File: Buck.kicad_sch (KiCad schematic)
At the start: 6 parts, among them U1501 XL1509

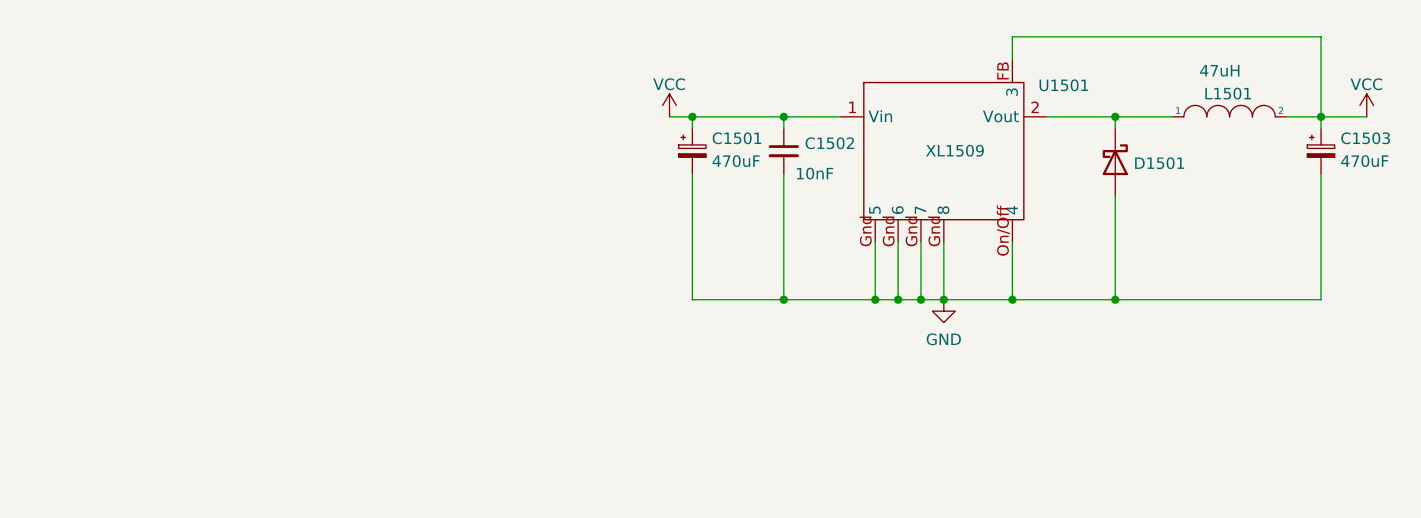
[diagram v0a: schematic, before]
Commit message: made additions to the project
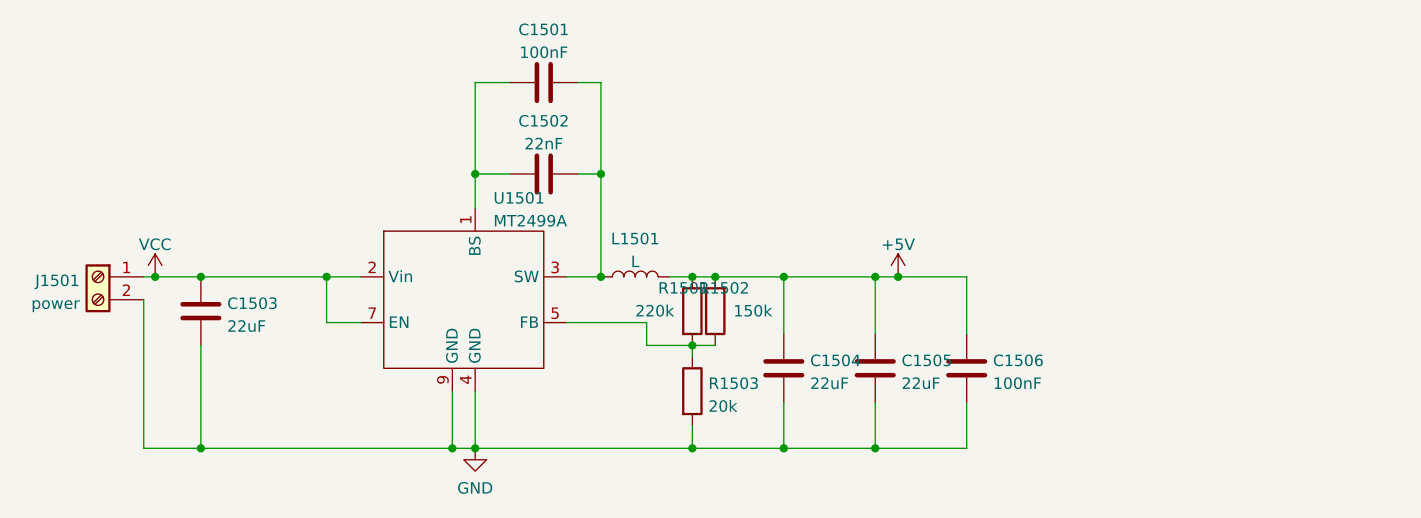
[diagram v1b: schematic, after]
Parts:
- removed C1501, C1503: 470uF, Capacitor_SMD:CP_Elec_8x10.5, symbol Device:C_Polarized_Small
- removed C1502: 10nF, Resistor_SMD:R_0805_2012Metric_Pad1.20x1.40mm_HandSolder, symbol Device:C_Small
- removed D1501: D_Schottky, Diode_SMD:D_SMA_Handsoldering, symbol Device:D_Schottky
- removed L1501: 47uH, Inductor_SMD:L_6.3x6.3_H3, symbol pspice:INDUCTOR
- removed U1501: XL1509, Package_SO:SOP-8_3.9x4.9mm_P1.27mm, symbol custom_bas:XL1509
- added C1501, C1506: 100nF, Capacitor_SMD:C_0402_1005Metric_Pad0.74x0.62mm_HandSolder, symbol Device:C
- added C1502: 22nF, Capacitor_SMD:C_0402_1005Metric_Pad0.74x0.62mm_HandSolder, symbol Device:C
- added C1503, C1504, C1505: 22uF, Capacitor_SMD:C_0603_1608Metric_Pad1.08x0.95mm_HandSolder, symbol Device:C
- added J1501: power, TerminalBlock_Phoenix:TerminalBlock_Phoenix_MKDS-1,5-2-5.08_1x02_P5.08mm_Horizontal, symbol Connector:Screw_Terminal_01x02
- added L1501: L, Inductor_SMD:L_Bourns-SRU8028_8.0x8.0mm, symbol Device:L
- added R1501: 220k, Resistor_SMD:R_0603_1608Metric_Pad0.98x0.95mm_HandSolder, symbol Device:R
- added R1502: 150k, Resistor_SMD:R_0603_1608Metric_Pad0.98x0.95mm_HandSolder, symbol Device:R
- added R1503: 20k, Resistor_SMD:R_0603_1608Metric_Pad0.98x0.95mm_HandSolder, symbol Device:R
- added U1501: MT2499A, Package_SO:TI_SO-PowerPAD-8, symbol custom_kicad_lib_sk:MT499A
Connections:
- net GND: now also C1503.2, C1504.2, C1505.2, C1506.2, J1501.2 (Pin_2), R1503.2, U1501.4 (GND), U1501.9 (GND)
- net VCC: now also C1503.1, J1501.1 (Pin_1), U1501.2 (Vin), U1501.7 (EN)
- new net: R1501.2, R1502.1, R1503.1, U1501.5 (FB)
- new net: C1501.1, C1502.1, U1501.1 (BS)
- new net: C1501.2, C1502.2, L1501.1, U1501.3 (SW)
- new net +5V: C1504.1, C1505.1, C1506.1, L1501.2, R1501.1, R1502.2
